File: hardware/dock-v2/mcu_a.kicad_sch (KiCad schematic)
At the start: 29 parts, among them SW301 SW_Push, SW302 SW_Push, U301 RP2354A, Y301 12MHz

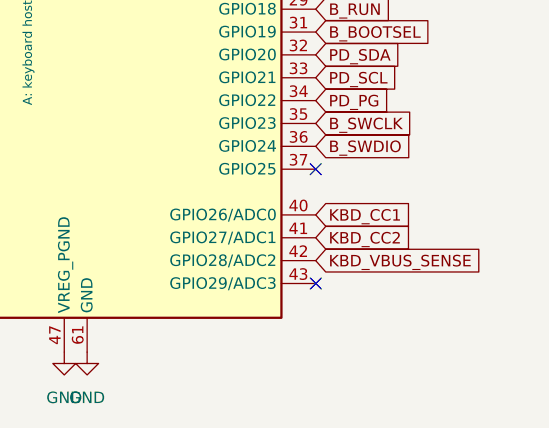
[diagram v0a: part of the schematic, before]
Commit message: Dock v2 schematic: user's fixes (snapshot)
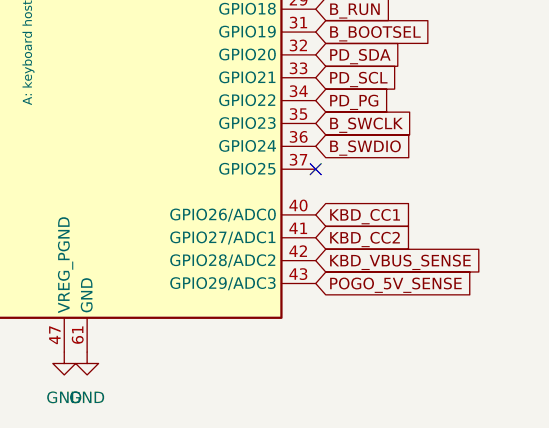
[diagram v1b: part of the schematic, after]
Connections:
- net POGO_5V_SENSE: now reaches U301.43 (GPIO29/ADC3)
- no-connect marks 10 -> 9
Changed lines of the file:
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@@
-	)
-	(no_connect
-		(at 209.55 157.48)
 	)
 	(no_connect
@@
 			(hide yes)
 			(show_name no)
+			(do_not_autoplace no)
+			(effects
+				(font
+					(size 1.27 1.27)
+				)
+				(justify left)
+			)
+		)
+	)
+	(global_label "POGO_5V_SENSE"
+		(shape input)
+		(at 209.55 157.48 0)
+		(fields_autoplaced yes)
+		(effects
+			(font
+				(size 1.27 1.27)
+			)
+			(justify left)
+		)
+		(property "Intersheetrefs" "${INTERSHEET_REFS}"
+			(at 228.017 157.48 0)
+			(hide yes)
+			(show_name no)
